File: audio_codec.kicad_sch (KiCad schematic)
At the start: 22 parts, among them J2 AudioOutput, J3 AudioInput, J4 AudioOutput, U2 WM8731SEDS, U5 TPA6110A2DGN

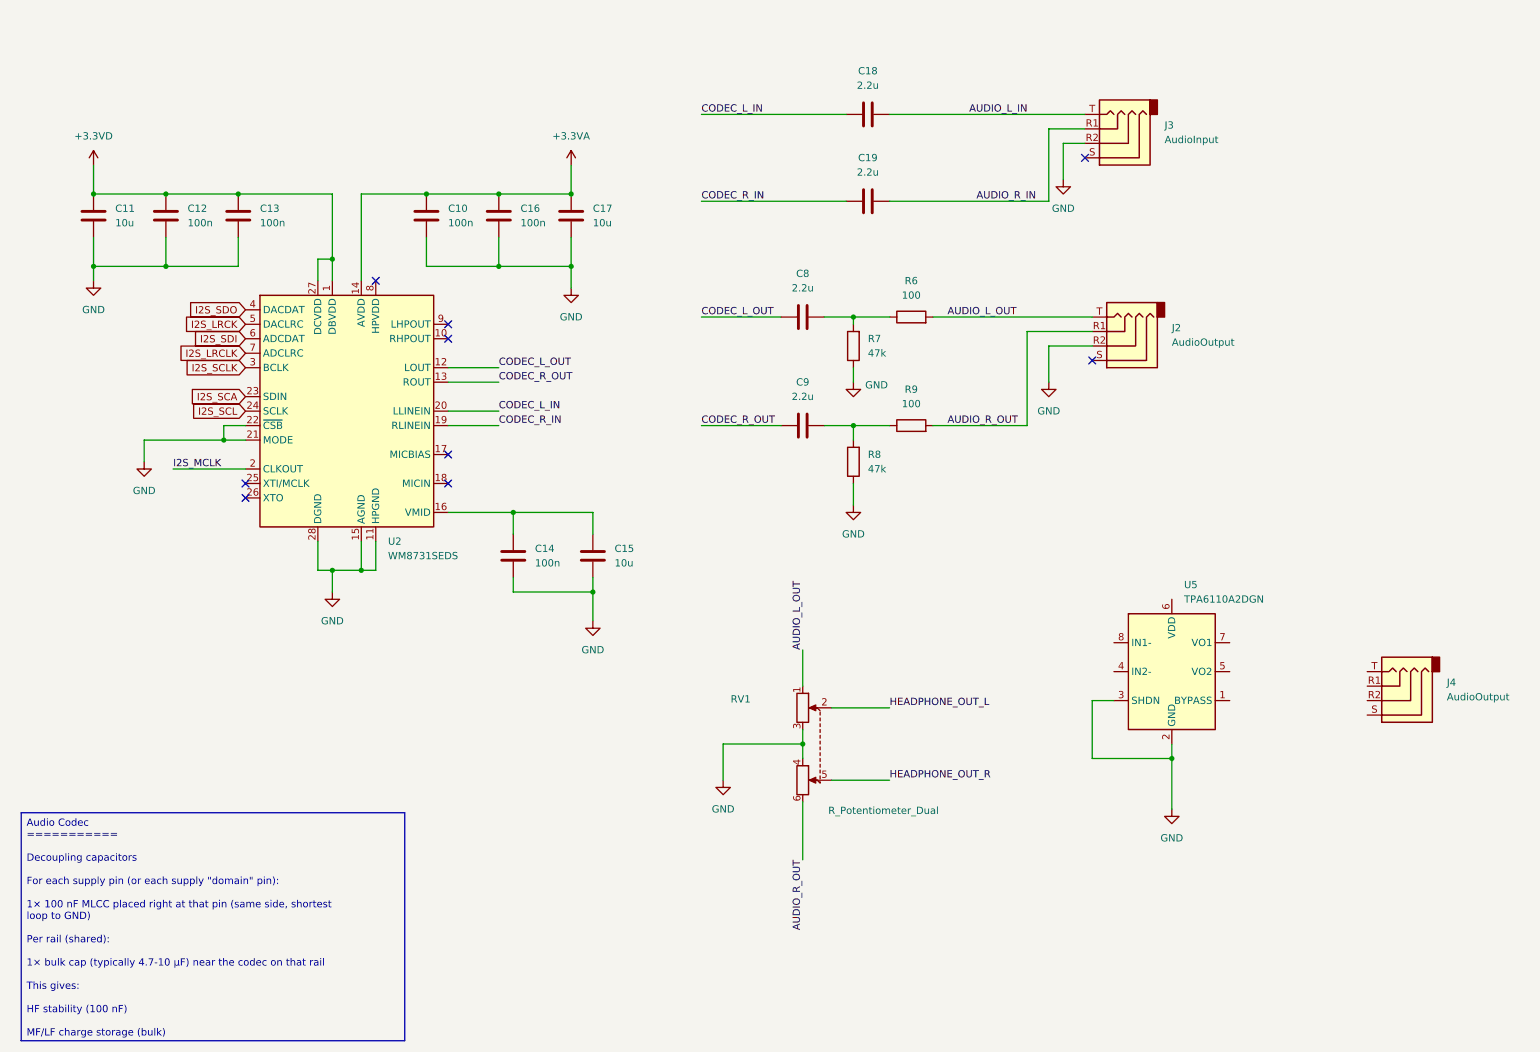
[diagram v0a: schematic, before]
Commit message: Audio schematic updated
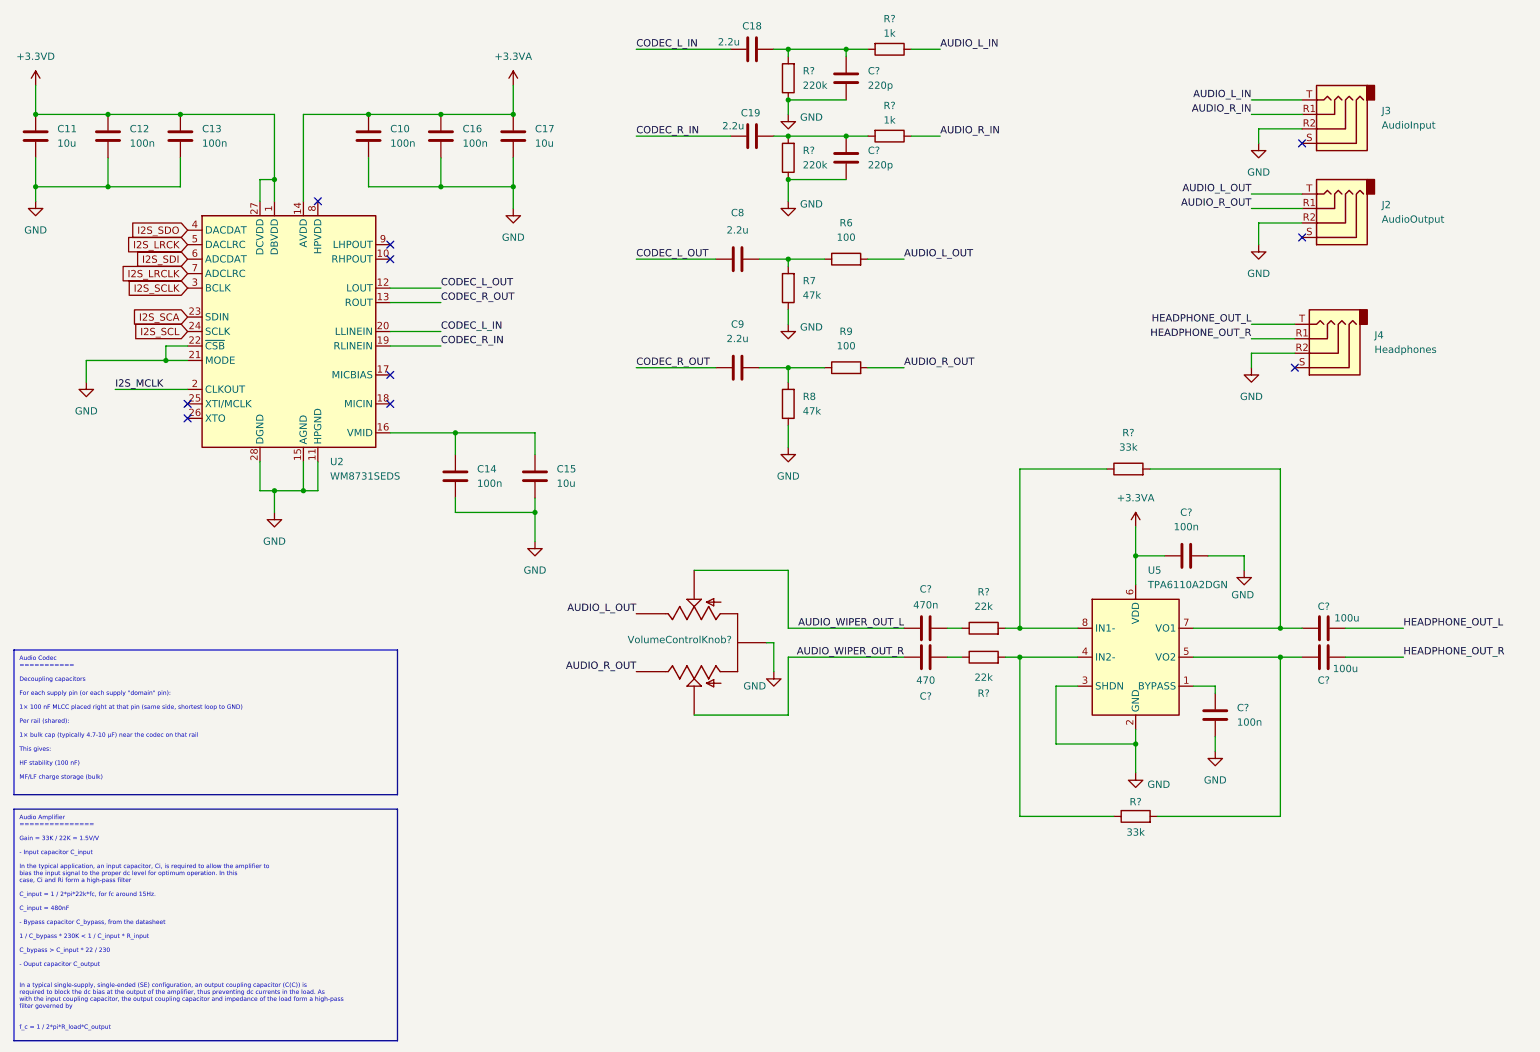
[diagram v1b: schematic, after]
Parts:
- removed RV1: R_Potentiometer_Dual, symbol Device:R_Potentiometer_Dual
- added C?: 470, symbol Device:C
- added C? (x2): 100n, symbol Device:C
- added C?: 470n, symbol Device:C
- added C? (x2): 220p, symbol Device:C
- added C? (x2): 100u, symbol Device:C
- added R? (x2): 33k, symbol Device:R
- added R? (x2): 220k, symbol Device:R
- added R? (x2): 22k, symbol Device:R
- added R? (x2): 1k, symbol Device:R
- added VolumeControlKnob?: ~, Galerna:RK10J12R0A0B, symbol Galerna:RK10J12R0A0B
- J4: value AudioOutput -> Headphones
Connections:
- net +3.3VA: now also U5.6 (VDD), C?.2
- net AUDIO_L_IN: now also R?.1; no longer C18.1
- net AUDIO_L_OUT: now also VolumeControlKnob?.4 (P4)
- net AUDIO_R_IN: now also R?.1; no longer C19.1
- net AUDIO_R_OUT: now also VolumeControlKnob?.5 (P5)
- net GND: now also J4.R2, C?.1, C?.1, C?.2, C?.2, R?.1, R?.1, VolumeControlKnob?.1 (P1)
- net HEADPHONE_OUT_L: now also J4.T, C?.2
- net HEADPHONE_OUT_R: now also J4.R1, C?.2
- net at U5.1 (BYPASS): now also C?.2
- net at U5.4 (IN2-): now also R?.1, R?.2
- net at U5.5 (VO2): now also C?.1, R?.2
- net at U5.7 (VO1): now also C?.1, R?.2
- net at U5.8 (IN1-): now also R?.1, R?.2
- new net: C?.2, R?.1 (x2)
- new net: C18.1, C?.1, R?.2, R?.2
- new net: C19.1, C?.1, R?.2, R?.2
- new net AUDIO_WIPER_OUT_L: C?.1, VolumeControlKnob?.3 (P3)
- new net AUDIO_WIPER_OUT_R: C?.1, VolumeControlKnob?.2 (P2)
- no-connect marks 9 -> 10
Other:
- moved on the sheet: C10, C11, C12, C13, C14, C15, C16, C17, C18, C19, C8, C9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
